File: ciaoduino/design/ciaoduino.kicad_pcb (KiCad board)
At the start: 2 copper layers, 8 parts, among them P1 ICSP, SW1 SW_PUSH, SW2 SW_PUSH, X1 CRYSTAL_SMD

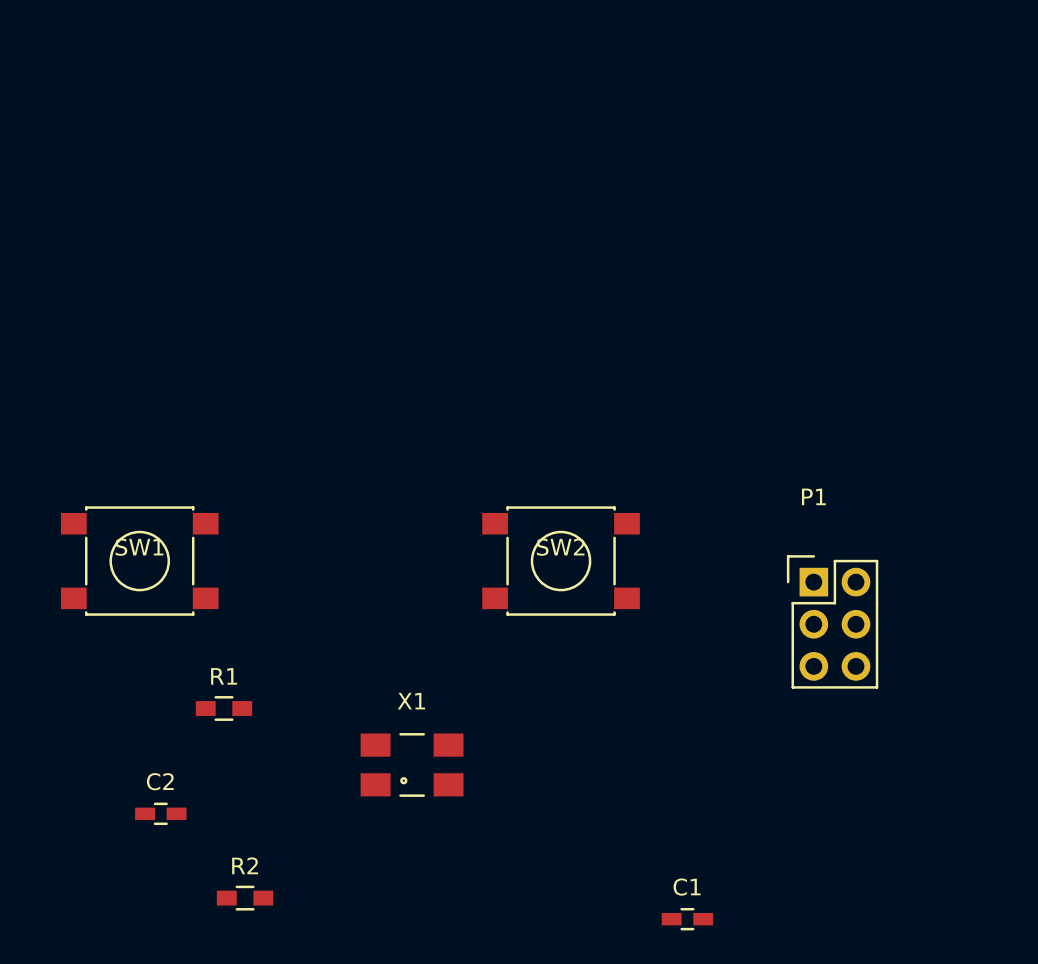
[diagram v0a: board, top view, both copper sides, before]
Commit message: Make more realistic board.
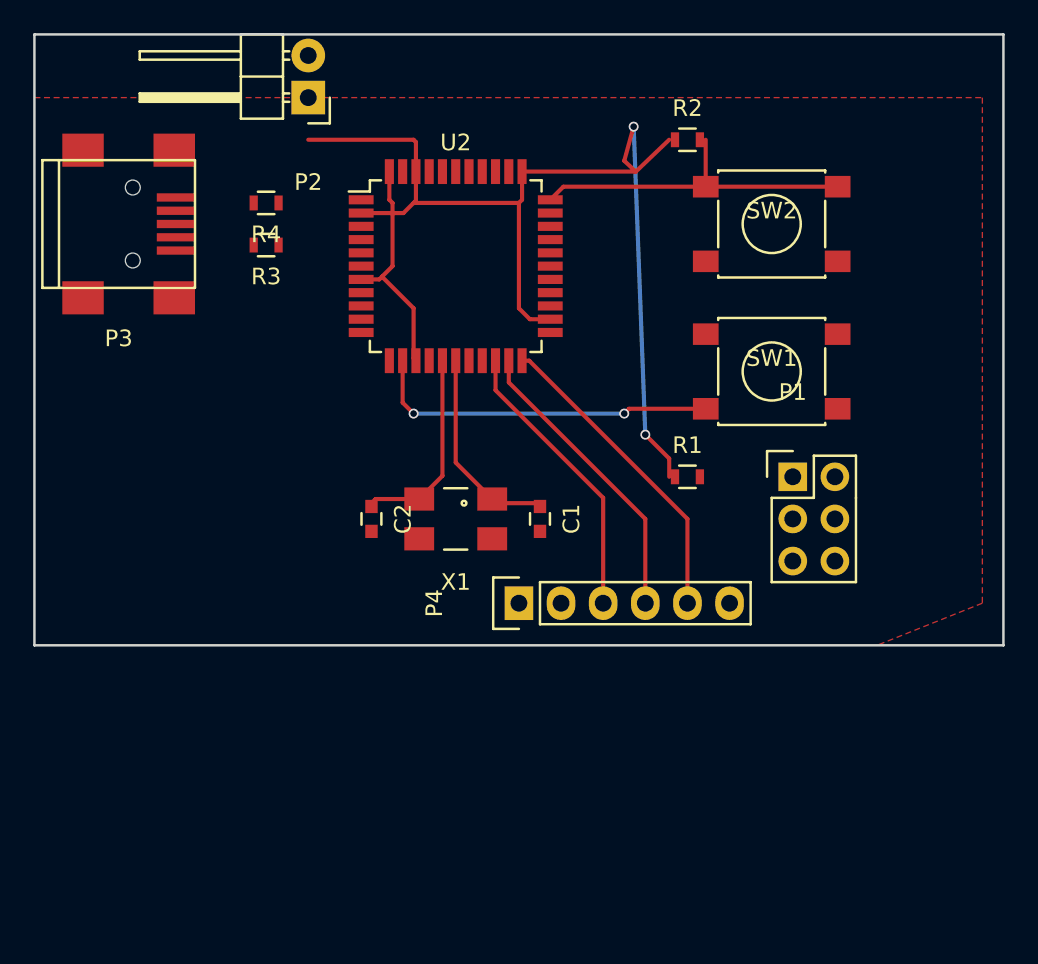
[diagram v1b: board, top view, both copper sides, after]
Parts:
- added P2: CONN_01X02, Pin_Headers:Pin_Header_Angled_1x02, F.Cu at (142.2, 64.8)
- added P3: USB_OTG, Connect:USB_Mini-B, F.Cu at (130.8, 72.4)
- added P4: CONN_01X06, Pin_Headers:Pin_Header_Straight_1x06, F.Cu at (154.9, 95.2)
- added R3: R, Resistors_SMD:R_0603, F.Cu at (139.7, 73.7)
- added R4: R, Resistors_SMD:R_0603, F.Cu at (139.7, 71.1)
- added U2: ATmega32U4-AU, Housings_QFP:TQFP-44_10x10mm_Pitch0.8mm, F.Cu at (151.1, 74.9)
- C1, C2: footprint Capacitors_SMD:C_0603_HandSoldering -> Capacitors_SMD:C_0603
- R1, R2: footprint Resistors_SMD:R_0603_HandSoldering -> Resistors_SMD:R_0603
- moved R2 52.9 mm to (165.1, 67.3)
- moved SW1 39.8 mm to (170.2, 81.3)
- moved R1 31.2 mm to (165.1, 87.6)
- moved C1 25.7 mm to (156.2, 90.2), turned to 270 degrees
- moved SW2 24.0 mm to (170.2, 72.4)
- moved C2 21.8 mm to (146.1, 90.2), turned to 270 degrees
- moved X1 15.1 mm to (151.1, 90.2), turned to 180 degrees
- moved P1 6.48 mm to (171.4, 87.6)
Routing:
- net VCC: track 0.00 -> 78.9 mm, vias 0 -> 2
- net Net-(R1-Pad2): track 0.00 -> 21.2 mm, vias 0 -> 2
- net Net-(R2-Pad2): track 0.00 -> 20.5 mm
- net usart_cts: track 0.00 -> 19.0 mm
- net usart_tx: track 0.00 -> 18.0 mm
- net usart_rx: track 0.00 -> 17.3 mm
- net Net-(C1-Pad1): track 0.00 -> 12.2 mm
- net Net-(C2-Pad1): track 0.00 -> 11.9 mm
- added copper zone on F.Cu, net GND
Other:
- board outline added: 58.4 x 36.8 mm
